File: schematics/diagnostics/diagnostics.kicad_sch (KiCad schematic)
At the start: 10 parts, among them J2 Conn_01x06_Socket, J3 Conn_02x04_Odd_Even

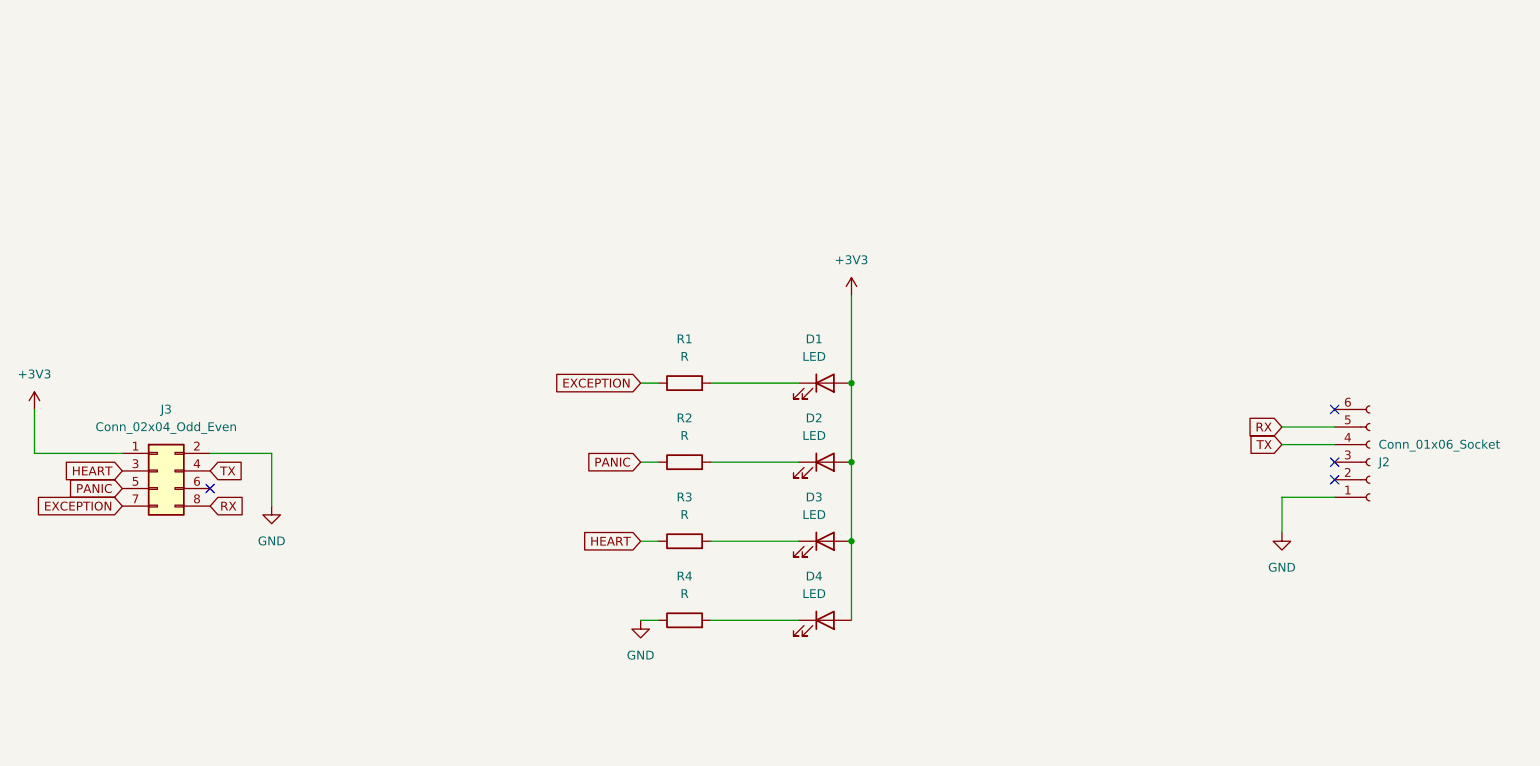
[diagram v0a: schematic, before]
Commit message: Signed-off-by: Ray33ee <30669752+ray33ee@users.noreply.github.com>
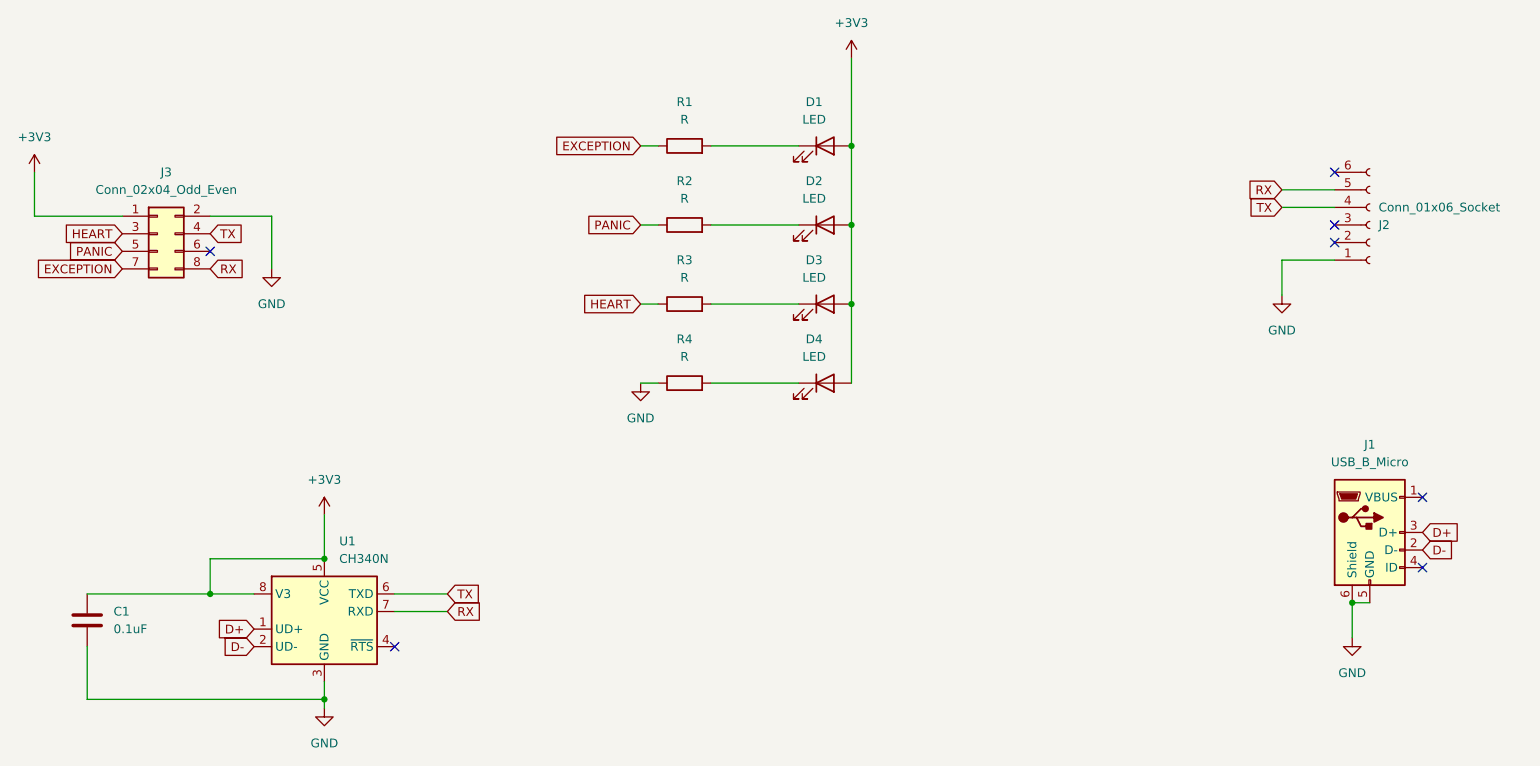
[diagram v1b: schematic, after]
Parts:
- added C1: 0.1uF, Capacitor_SMD:C_1206_3216Metric_Pad1.33x1.80mm_HandSolder, symbol Device:C
- added J1: USB_B_Micro, symbol Connector:USB_B_Micro
- added U1: CH340N, Package_SO:SOP-8_3.9x4.9mm_P1.27mm, symbol Interface_USB:CH340N
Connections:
- net +3V3: now also C1.1, U1.5 (VCC), U1.8 (V3)
- net GND: now also C1.2, J1.5 (GND), J1.6 (Shield), U1.3 (GND)
- net RX: now also U1.7 (RXD)
- net TX: now also U1.6 (TXD)
- new net D+: J1.3 (D+), U1.1 (UD+)
- new net D-: J1.2 (D-), U1.2 (UD-)
- no-connect marks 4 -> 7
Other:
- moved on the sheet: D1, D2, D3, D4, J2, J3, R1, R2, R3, R4
